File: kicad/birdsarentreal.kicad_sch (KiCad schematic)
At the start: 34 parts, among them J1 Adafruit Coil Jumper, J2 Adafruit Coil Jumper, J3 Adafruit Coil Jumper, J4 Adafruit Coil Jumper, Q2 NMOS, U9 MCP73831-2-OT

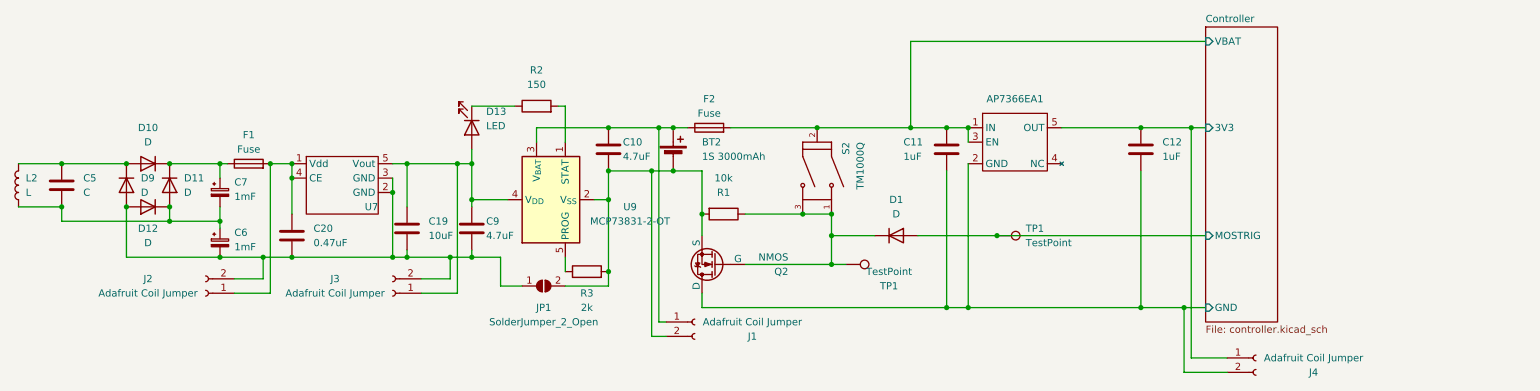
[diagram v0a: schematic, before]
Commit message: Make schematic pretty
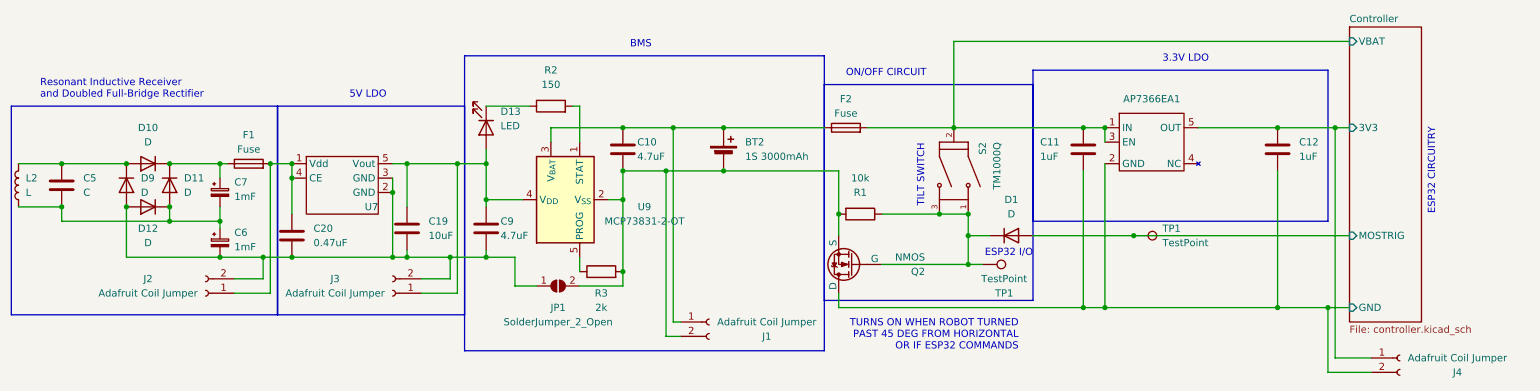
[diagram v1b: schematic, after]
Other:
- note added: "3.3V LDO"
- note added: "5V LDO"
- note added: "BMS"
- note added: "ESP32 CIRCUITRY"
- note added: "ESP32 I/O"
- note added: "ON/OFF CIRCUIT"
- note added: "Resonant Inductive Receiver and Doubled Full-Bridge Rectifier"
- note added: "TILT SWITCH"
- note added: "TURNS ON WHEN ROBOT TURNED PAST 45 DEG FROM HORIZONTAL OR IF ESP32 COMMANDS"
- moved on the sheet: AP7366EA1, BT2, C10, C11, C12, C9, D1, D13, F2, J1, J4, JP1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
